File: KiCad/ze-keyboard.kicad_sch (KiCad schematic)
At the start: 25 parts, among them J1 AVR-ISP-6, SW1 SW_Push, SW2 SW_Push_Reset, SW3 SW_Push, U1 ATmega32U4-A, U2 PRTR5V0U2X, Y1 Crystal_GND24_Small

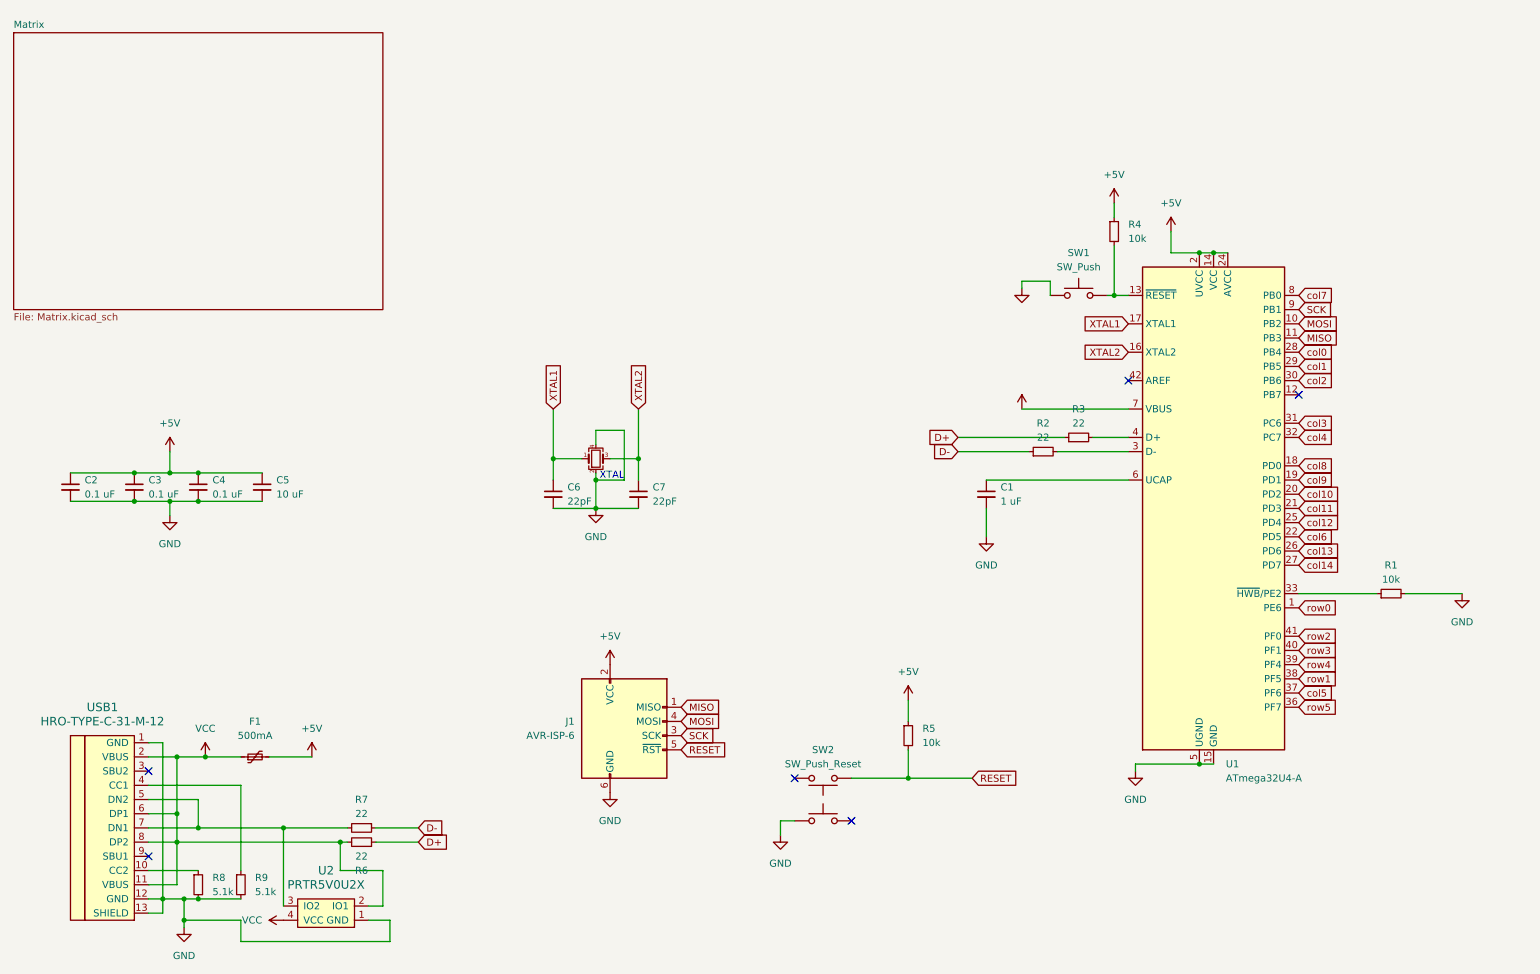
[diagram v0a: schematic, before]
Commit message: fix stuff... i forgot the other stuff i added
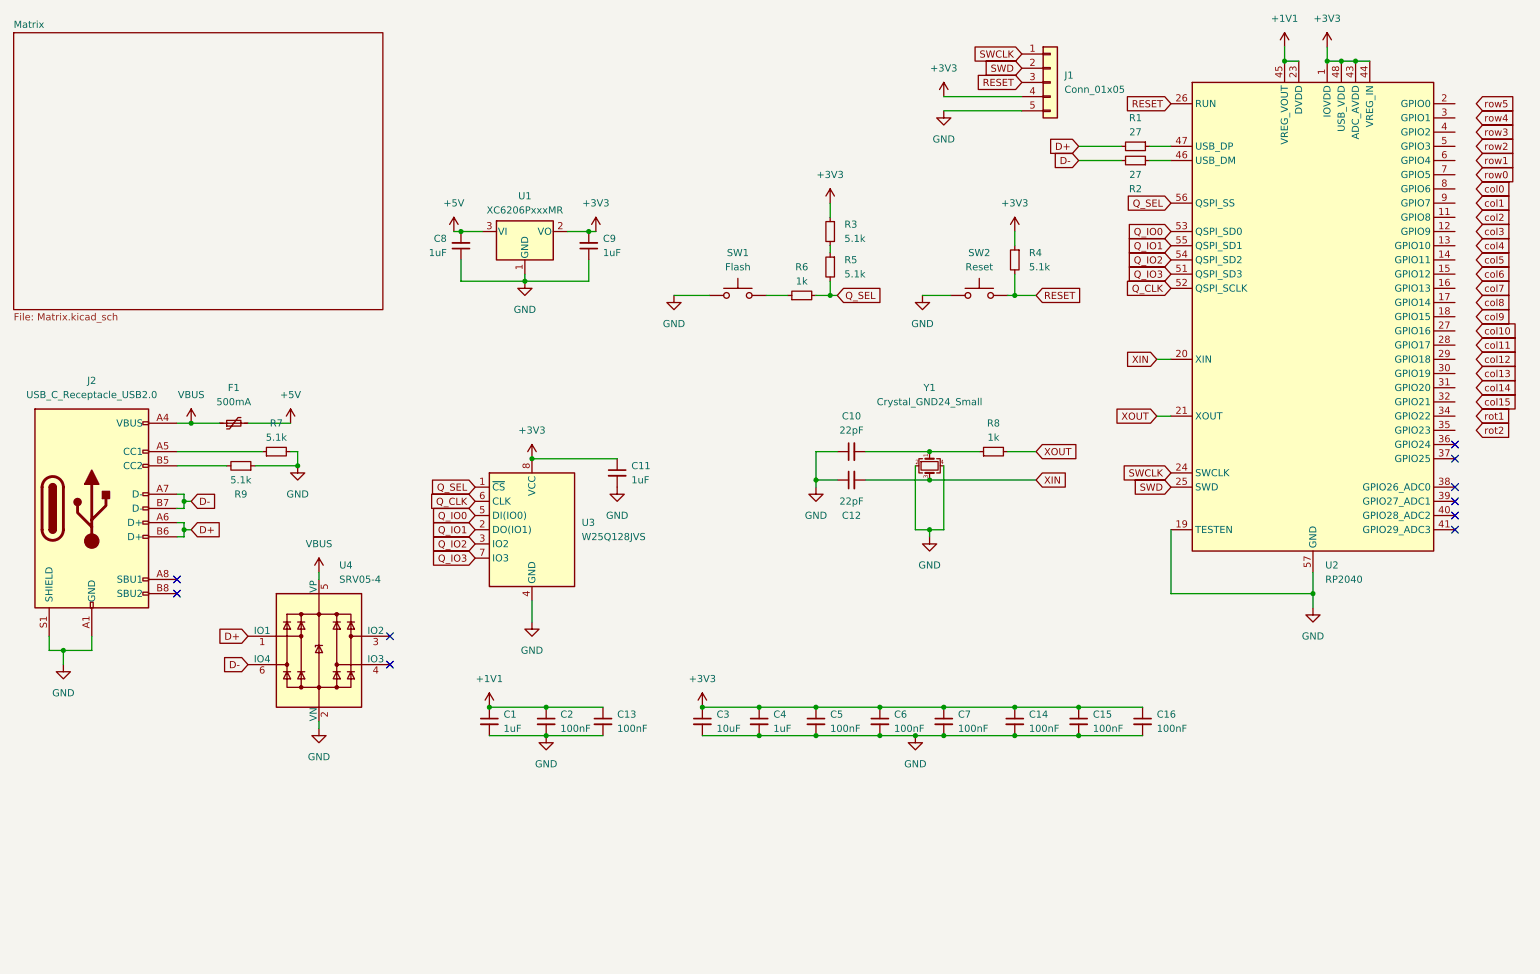
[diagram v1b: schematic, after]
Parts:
- removed J1: AVR-ISP-6, symbol Connector:AVR-ISP-6
- removed SW3: SW_Push, symbol Switch:SW_Push
- removed U1: ATmega32U4-A, Package_QFP:TQFP-44_10x10mm_P0.8mm, symbol MCU_Microchip_ATmega:ATmega32U4-A
- removed U2: PRTR5V0U2X, symbol random-keyboard-parts:PRTR5V0U2X
- removed USB1: HRO-TYPE-C-31-M-12, symbol Type-C:HRO-TYPE-C-31-M-12
- added C10, C12: 22pF, Capacitor_SMD:C_0402_1005Metric, symbol Device:C_Small
- added C11, C8, C9: 1uF, Capacitor_SMD:C_0402_1005Metric, symbol Device:C_Small
- added C13, C14, C15, C16: 100nF, Capacitor_SMD:C_0402_1005Metric, symbol Device:C_Small
- added J1: Conn_01x05, Connector_PinHeader_2.54mm:PinHeader_1x05_P2.54mm_Vertical, symbol Connector_Generic:Conn_01x05
- added J2: USB_C_Receptacle_USB2.0, Connector_USB:USB_C_Receptacle_HRO_TYPE-C-31-M-12, symbol Connector:USB_C_Receptacle_USB2.0
- added U1: XC6206PxxxMR, Package_TO_SOT_SMD:SOT-23-3, symbol Regulator_Linear:XC6206PxxxMR
- added U2: RP2040, Package_DFN_QFN:QFN-56-1EP_7x7mm_P0.4mm_EP3.2x3.2mm, symbol MCU_RaspberryPi:RP2040
- added U3: W25Q128JVS, Package_SO:SOIC-8_5.23x5.23mm_P1.27mm, symbol Memory_Flash:W25Q128JVS
- added U4: SRV05-4, PCM_marbastlib-various:SOT-23-6-routable, symbol PCM_marbastlib-various:SRV05-4
- C1: value 1 uF -> 1uF; footprint (none) -> Capacitor_SMD:C_0402_1005Metric
- C2: value 0.1 uF -> 100nF; footprint (none) -> Capacitor_SMD:C_0402_1005Metric
- C3: value 0.1 uF -> 10uF; footprint (none) -> Capacitor_SMD:C_0603_1608Metric
- C4: value 0.1 uF -> 1uF; footprint (none) -> Capacitor_SMD:C_0402_1005Metric
- C5: value 10 uF -> 100nF; footprint (none) -> Capacitor_SMD:C_0402_1005Metric
- C6, C7: value 22pF -> 100nF; footprint (none) -> Capacitor_SMD:C_0402_1005Metric
- F1: footprint (none) -> Fuse:Fuse_1206_3216Metric
- R1: value 10k -> 27; footprint (none) -> Resistor_SMD:R_0402_1005Metric
- R2: value 22 -> 27; footprint (none) -> Resistor_SMD:R_0402_1005Metric
- R3, R7: value 22 -> 5.1k; footprint (none) -> Resistor_SMD:R_0402_1005Metric
- R4, R5: value 10k -> 5.1k; footprint (none) -> Resistor_SMD:R_0402_1005Metric
- R6: value 22 -> 1k; footprint (none) -> Resistor_SMD:R_0402_1005Metric
- R8: value 5.1k -> 1k; footprint (none) -> Resistor_SMD:R_0402_1005Metric
- R9: footprint (none) -> Resistor_SMD:R_0402_1005Metric
- SW1: value SW_Push -> Flash; footprint (none) -> Button_Switch_SMD:SW_SPST_TL3342
- SW2: value SW_Push_Reset -> Reset; footprint (none) -> Button_Switch_SMD:SW_SPST_TL3342
- Y1: footprint (none) -> Crystal:Crystal_SMD_3225-4Pin_3.2x2.5mm
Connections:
- net +5V: now also C8.2, U1.3 (VI); no longer C2.1, C3.1, C4.1, C5.1, R4.1, R5.1
- net D+: now also R1.2, J2.A6 (D+), J2.B6 (D+), U4.1 (IO1); no longer R3.1, R6.1
- net D-: now also R2.2, J2.A7 (D-), J2.B7 (D-), U4.6 (IO4); no longer R2.1, R7.1
- net GND: now also R7.2, R9.1, SW2.1, C10.1, C11.2, C12.1, C13.2, C14.2, C15.2, C16.2, C8.1, C9.1, J1.5 (Pin_5), J2.A1 (GND), J2.A12 (GND), J2.B1 (GND), J2.B12 (GND), J2.S1 (SHIELD), U1.1 (GND), U2.19 (TESTEN), U2.57 (GND), U3.4 (GND), U4.2 (VN); no longer R1.2, R8.2, R9.2
- net RESET: now also R4.2, SW2.2, J1.3 (Pin_3), U2.26 (RUN); no longer R5.2, SW2.1
- net at R8.1: now also Y1.1, C10.2
- net at R3.2: now also R5.1
- net at R1.1: now also U2.47 (USB_DP)
- net at SW1.2: now also R6.1; no longer R4.2
- net +1V1: now reaches C1.1
- net +1V1: now also C2.1, C13.1, U2.23 (DVDD), U2.45 (VREG_VOUT), U2.50 (DVDD)
- net VCC renamed Q_SEL
- net Q_SEL: now also R5.2, U2.56 (QSPI_SS), U3.1 (~{CS}); no longer F1.1
- net XTAL1 renamed +3V3
- net +3V3: now also C3.1, C4.1, C5.1, C7.1, R3.1, R4.1, C11.1, C14.1, C15.1, C16.1, C9.2, J1.4 (Pin_4), U1.2 (VO), U2.1 (IOVDD), U2.10 (IOVDD), U2.22 (IOVDD), U2.33 (IOVDD), U2.42 (IOVDD), U2.43 (ADC_AVDD), U2.44 (VREG_IN), U2.48 (USB_VDD), U2.49 (IOVDD), U3.8 (VCC); no longer Y1.1
- net XTAL2 renamed XIN
- net XIN: now also C12.2, U2.20 (XIN); no longer C7.1
- new net: R2.1, U2.46 (USB_DM)
- new net: J2.B5 (CC2), R9.2
- new net: J2.A5 (CC1), R7.1
- new net Q_CLK: U2.52 (QSPI_SCLK), U3.6 (CLK)
- new net Q_IO0: U2.53 (QSPI_SD0), U3.5 (DI(IO0))
- new net Q_IO1: U2.55 (QSPI_SD1), U3.2 (DO(IO1))
- new net Q_IO2: U2.54 (QSPI_SD2), U3.3 (IO2)
- new net Q_IO3: U2.51 (QSPI_SD3), U3.7 (IO3)
- new net SWCLK: J1.1 (Pin_1), U2.24 (SWCLK)
- new net SWD: J1.2 (Pin_2), U2.25 (SWD)
- new net VBUS: F1.1, J2.A4 (VBUS), J2.A9 (VBUS), J2.B4 (VBUS), J2.B9 (VBUS), U4.5 (VP)
- new net XOUT: R8.2, U2.21 (XOUT)
- no-connect marks 6 -> 10
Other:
- note removed: "XTAL"

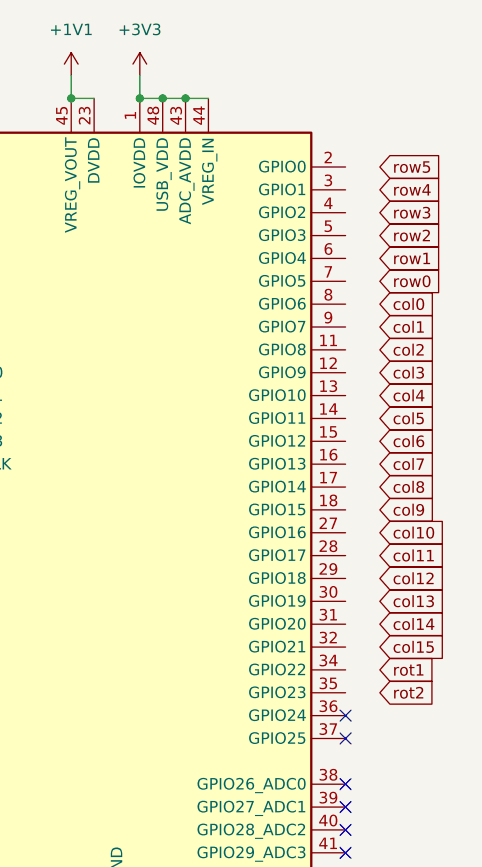
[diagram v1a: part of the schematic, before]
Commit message: do some tracing
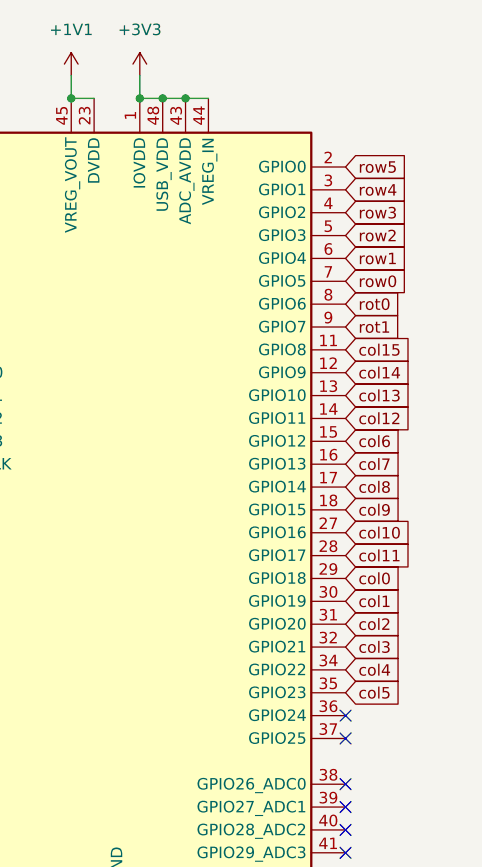
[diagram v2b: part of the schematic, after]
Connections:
- net col0: now also U2.29 (GPIO18)
- net col1: now also U2.30 (GPIO19)
- net col10: now also U2.27 (GPIO16)
- net col11: now also U2.28 (GPIO17)
- net col12: now also U2.14 (GPIO11)
- net col13: now also U2.13 (GPIO10)
- net col14: now also U2.12 (GPIO9)
- net col15: now also U2.11 (GPIO8)
- net col2: now also U2.31 (GPIO20)
- net col3: now also U2.32 (GPIO21)
- net col4: now also U2.34 (GPIO22)
- net col5: now also U2.35 (GPIO23)
- net col6: now also U2.15 (GPIO12)
- net col7: now also U2.16 (GPIO13)
- net col8: now also U2.17 (GPIO14)
- net col9: now also U2.18 (GPIO15)
- net rot1: now also U2.9 (GPIO7)
- net row0: now also U2.7 (GPIO5)
- net row1: now also U2.6 (GPIO4)
- net row2: now also U2.5 (GPIO3)
- net row3: now also U2.4 (GPIO2)
- net row4: now also U2.3 (GPIO1)
- net row5: now also U2.2 (GPIO0)
- net rot0: now reaches U2.8 (GPIO6)

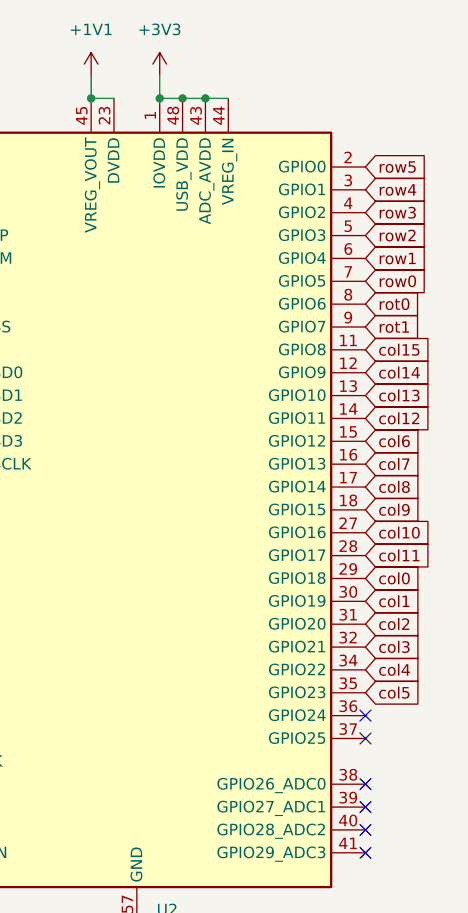
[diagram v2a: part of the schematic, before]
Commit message: finish pcb
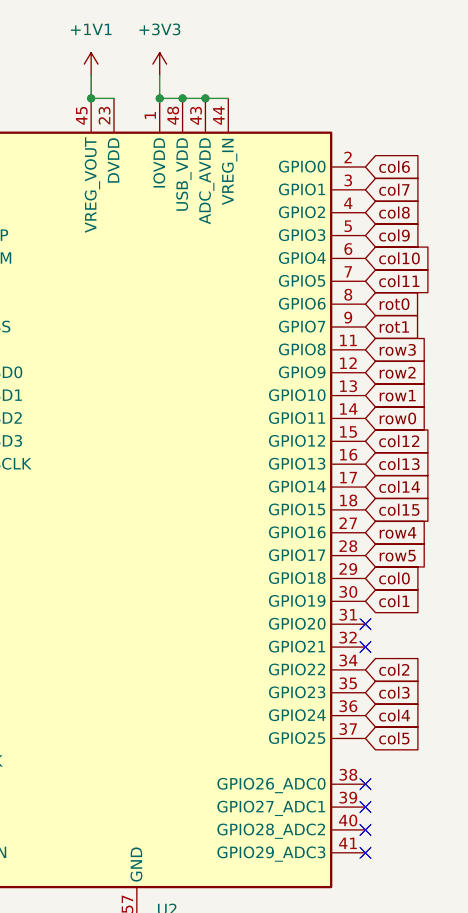
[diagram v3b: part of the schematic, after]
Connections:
- net col10: now also U2.6 (GPIO4); no longer U2.27 (GPIO16)
- net col11: now also U2.7 (GPIO5); no longer U2.28 (GPIO17)
- net col12: now also U2.15 (GPIO12); no longer U2.14 (GPIO11)
- net col13: now also U2.16 (GPIO13); no longer U2.13 (GPIO10)
- net col14: now also U2.17 (GPIO14); no longer U2.12 (GPIO9)
- net col15: now also U2.18 (GPIO15); no longer U2.11 (GPIO8)
- net col2: now also U2.34 (GPIO22); no longer U2.31 (GPIO20)
- net col3: now also U2.35 (GPIO23); no longer U2.32 (GPIO21)
- net col4: now also U2.36 (GPIO24); no longer U2.34 (GPIO22)
- net col5: now also U2.37 (GPIO25); no longer U2.35 (GPIO23)
- net col6: now also U2.2 (GPIO0); no longer U2.15 (GPIO12)
- net col7: now also U2.3 (GPIO1); no longer U2.16 (GPIO13)
- net col8: now also U2.4 (GPIO2); no longer U2.17 (GPIO14)
- net col9: now also U2.5 (GPIO3); no longer U2.18 (GPIO15)
- net row0: now also U2.14 (GPIO11); no longer U2.7 (GPIO5)
- net row1: now also U2.13 (GPIO10); no longer U2.6 (GPIO4)
- net row2: now also U2.12 (GPIO9); no longer U2.5 (GPIO3)
- net row3: now also U2.11 (GPIO8); no longer U2.4 (GPIO2)
- net row4: now also U2.27 (GPIO16); no longer U2.3 (GPIO1)
- net row5: now also U2.28 (GPIO17); no longer U2.2 (GPIO0)

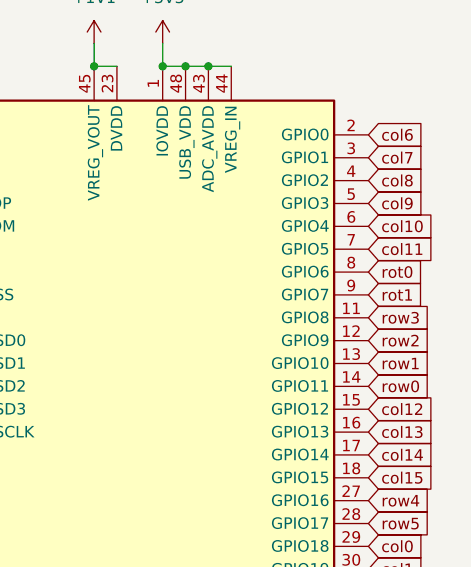
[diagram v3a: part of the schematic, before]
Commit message: some changes, a bit more jlcpcb stuff
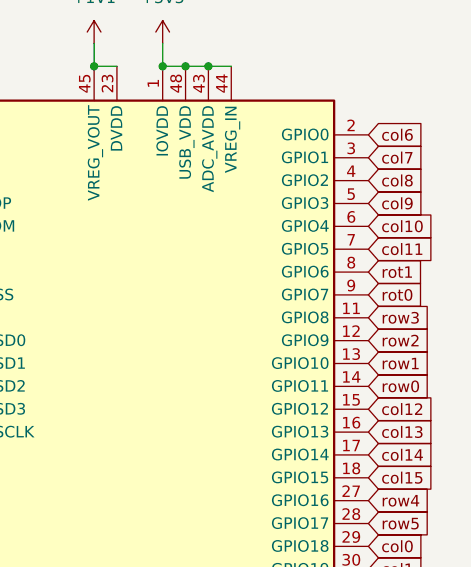
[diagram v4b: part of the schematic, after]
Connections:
- net rot0: now also U2.9 (GPIO7); no longer U2.8 (GPIO6)
- net rot1: now also U2.8 (GPIO6); no longer U2.9 (GPIO7)
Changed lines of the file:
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@@
     )
   )
-  (global_label "rot1" (shape input) (at 275.59 46.99 0) (fields_autoplaced)
+  (global_label "rot1" (shape input) (at 275.59 44.45 0) (fields_autoplaced)
     (effects (font (size 1.27 1.27)) (justify left))
-    (property "Intersheetrefs" "${INTERSHEET_REFS}" (at 282.4456 46.99 0)
+    (property "Intersheetrefs" "${INTERSHEET_REFS}" (at 282.4456 44.45 0)
       (effects (font (size 1.27 1.27)) (justify left) hide)
     )
@@
     )
   )
-  (global_label "rot0" (shape input) (at 275.59 44.45 0) (fields_autoplaced)
+  (global_label "rot0" (shape input) (at 275.59 46.99 0) (fields_autoplaced)
     (effects (font (size 1.27 1.27)) (justify left))
-    (property "Intersheetrefs" "${INTERSHEET_REFS}" (at 282.4456 44.45 0)
+    (property "Intersheetrefs" "${INTERSHEET_REFS}" (at 282.4456 46.99 0)
       (effects (font (size 1.27 1.27)) (justify left) hide)
     )
